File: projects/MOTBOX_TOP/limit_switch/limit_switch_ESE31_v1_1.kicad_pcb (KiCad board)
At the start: 2 copper layers, 17.8 x 16.5 mm, 3 parts, among them J1 Conn_01x03, SW1 ESE31R11T, SW2 ESE31L11T

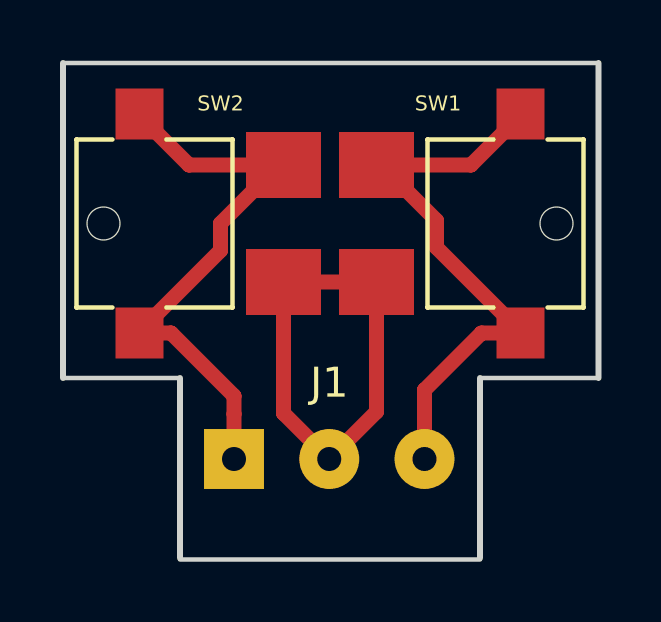
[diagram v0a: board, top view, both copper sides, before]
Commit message: Changes misc
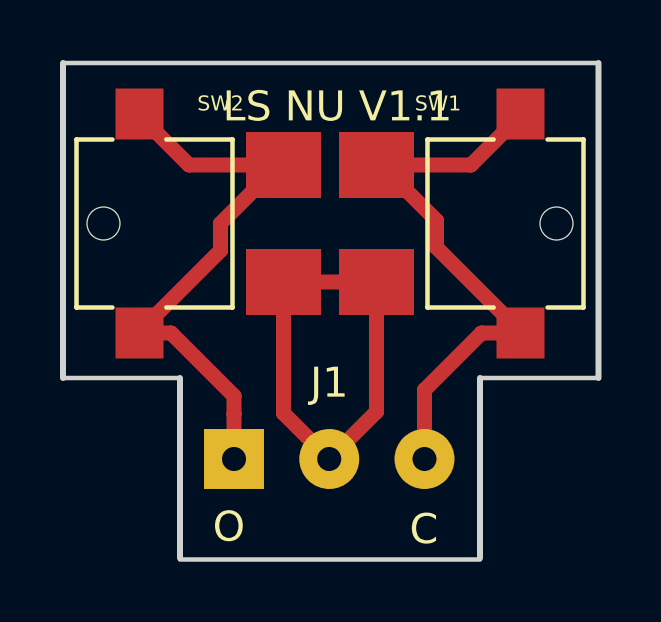
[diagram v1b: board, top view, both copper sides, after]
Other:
- board text added: "C"
- board text added: "LS NU V1.1"
- board text added: "O"
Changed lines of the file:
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@@
   (general
     (thickness 1.6)
-    (drawings 9)
+    (drawings 12)
     (tracks 29)
     (zones 0)
@@
     (47 F.CrtYd user)
     (48 B.Fab user)
-    (49 F.Fab user)
+    (49 F.Fab user hide)
   )
   (setup
@@
     (solder_mask_min_width 0.25)
     (aux_axis_origin 0 0)
-    (visible_elements FFFFFF7F)
+    (visible_elements FFFBFF7F)
     (pcbplotparams
       (layerselection 0x010fc_ffffffff)
@@
       (net 1 "Net-(J1-Pad3)"))
   )
+  (gr_text C (at 163.93 83.94) (layer F.SilkS)
+    (effects (font (size 1 1) (thickness 0.25)))
+  )
+  (gr_text O (at 157.43 83.86) (layer F.SilkS)
+    (effects (font (size 1 1) (thickness 0.25)))
+  )
+  (gr_text "LS NU V1.1" (at 161.05 69.85) (layer F.SilkS)
+    (effects (font (size 1 1) (thickness 0.25)))
+  )
   (gr_line (start 151.9 68.4) (end 169.75 68.4) (layer Edge.Cuts) (width 0.15))
